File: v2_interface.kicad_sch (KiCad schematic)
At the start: 27 parts, among them J10 Vref_Select, J14 AUX_Select, J15 DB25_Socket, J16 DE9_Socket, J5 Power, Q1 2N7002K, U1 MCP3424x-xSL, U11 MCP1501-20xCH, U12 MCP4922

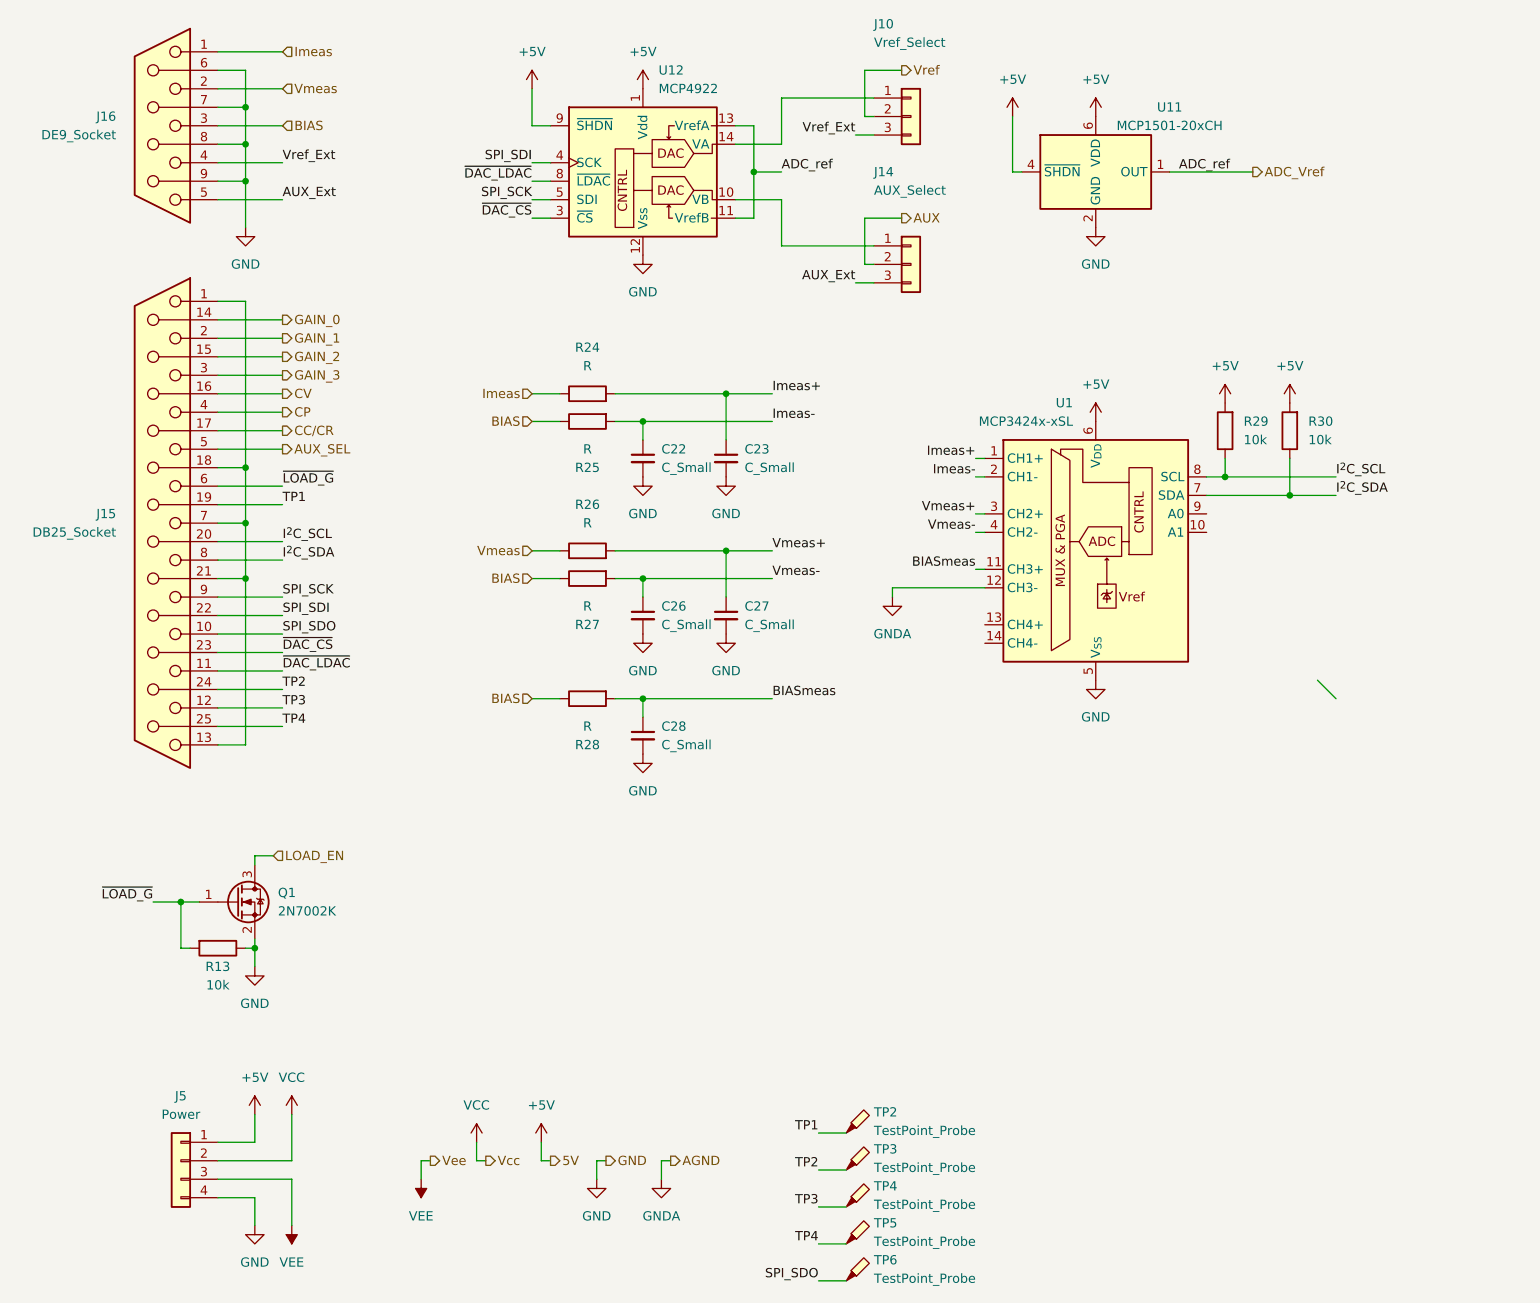
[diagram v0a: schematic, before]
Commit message: 電圧なににしよ
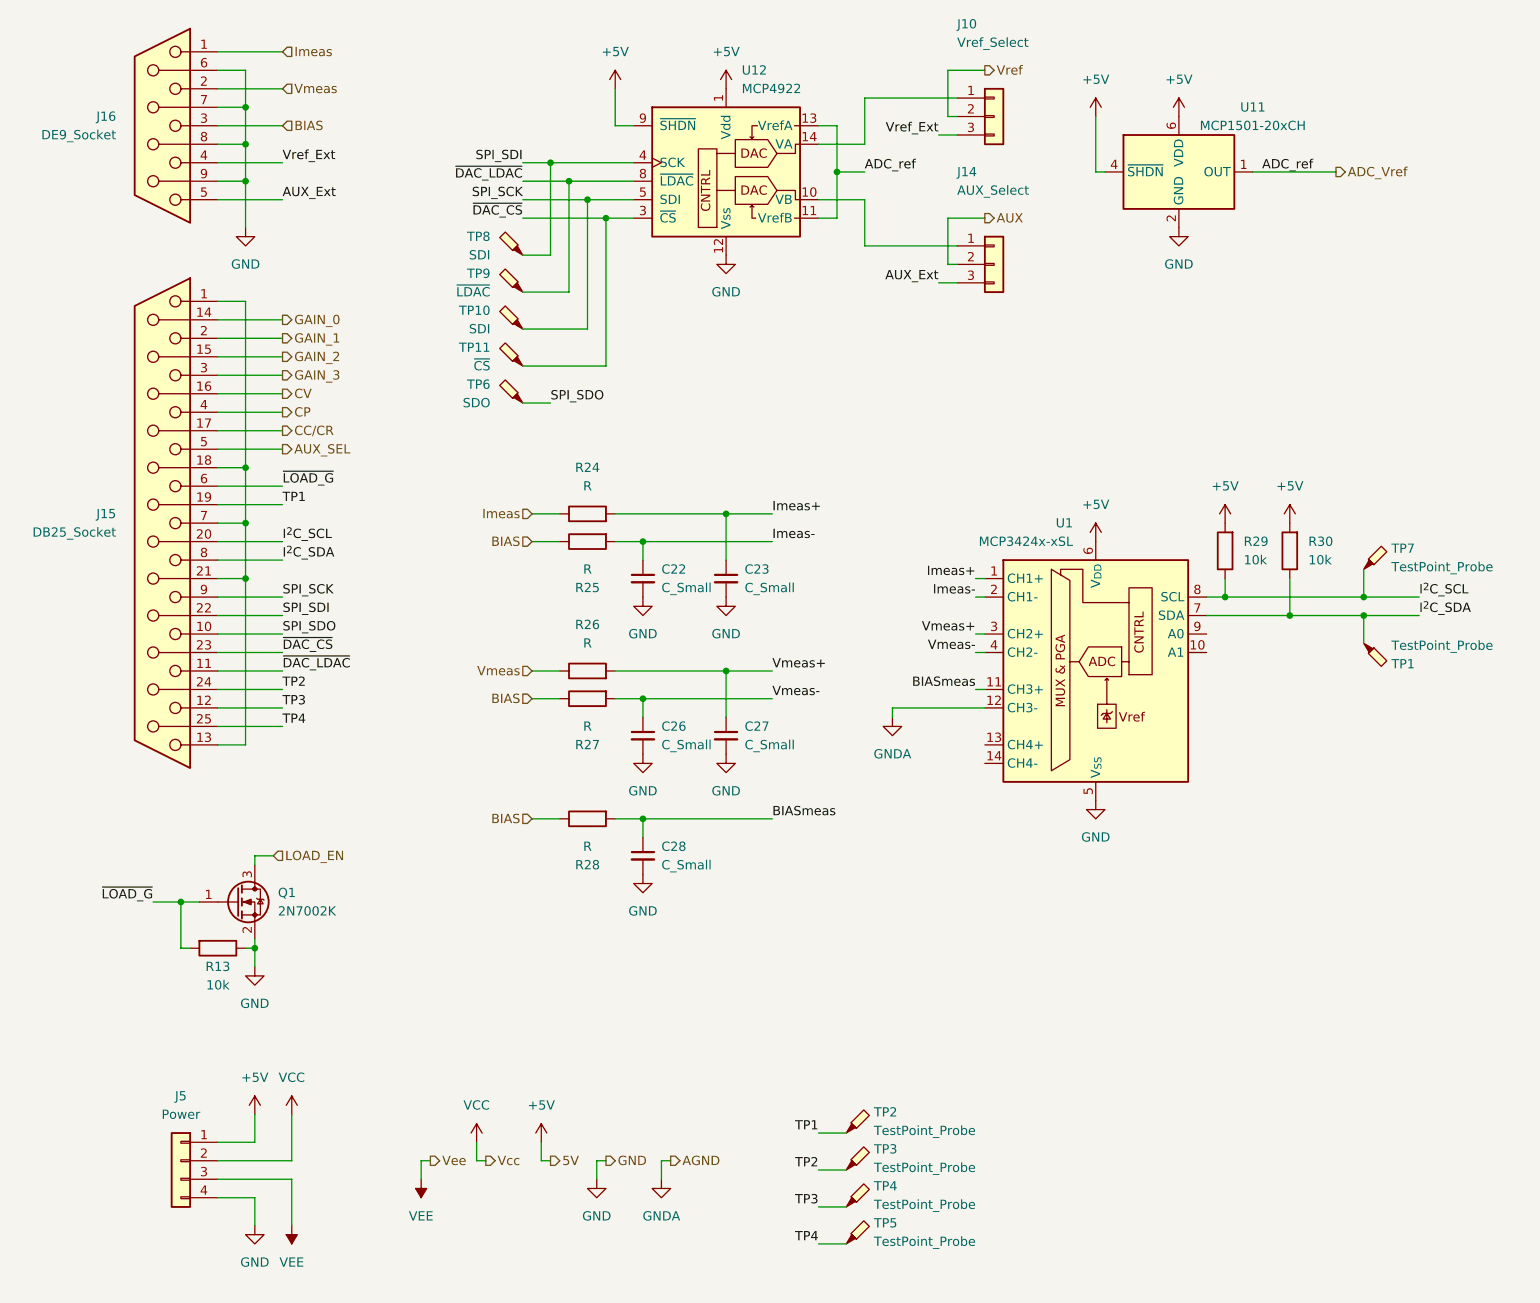
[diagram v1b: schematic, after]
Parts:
- added TP1, TP7: TestPoint_Probe, symbol Connector:TestPoint_Probe
- added TP10, TP8: SDI, symbol Connector:TestPoint_Probe
- added TP11: ~{CS}, symbol Connector:TestPoint_Probe
- added TP9: ~{LDAC}, symbol Connector:TestPoint_Probe
- TP6: value TestPoint_Probe -> SDO
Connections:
- net I^{2}C_SCL: now also TP7.1
- net I^{2}C_SDA: now also TP1.1
- net SPI_SCK: now also TP10.1
- net SPI_SDI: now also TP8.1
- net ~{DAC_CS}: now also TP11.1
- net ~{DAC_LDAC}: now also TP9.1
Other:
- moved on the sheet: C22, C23, C26, C27, C28, J10, J14, R24, R25, R26, R27, R28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
